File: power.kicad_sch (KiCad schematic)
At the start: 29 parts, among them Q1 DMN3008SFG, Q2 DMN3008SFG, U1 AP33771, U2 AP62150WU, U5 MCP1727T-3302E/SN

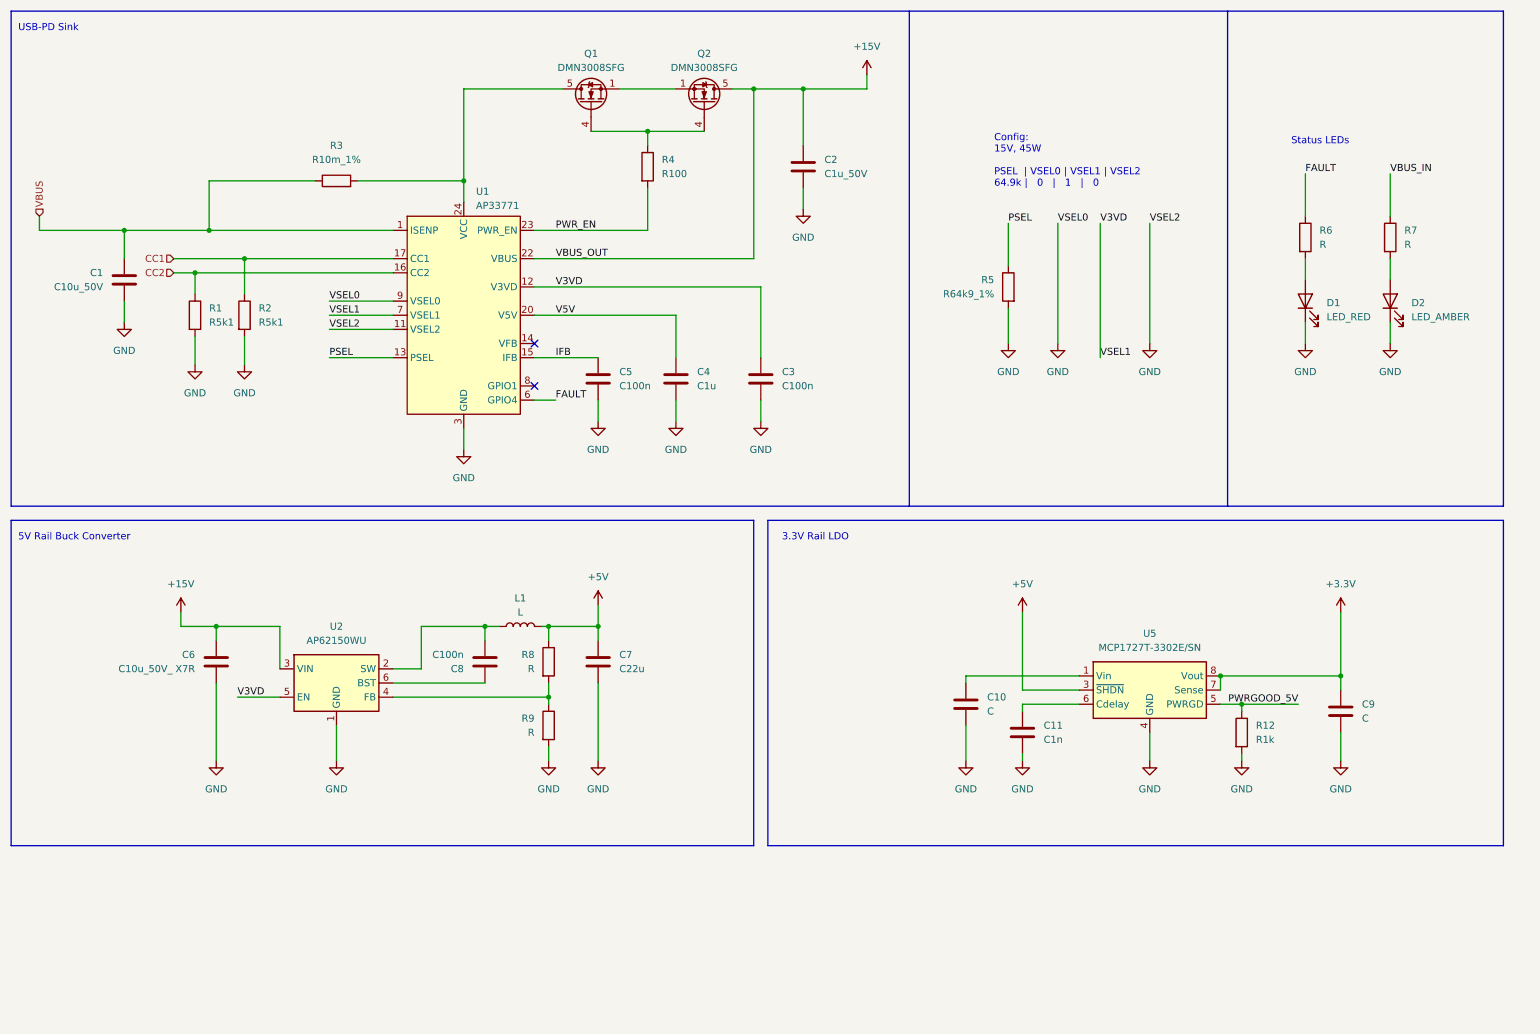
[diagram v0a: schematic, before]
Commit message: Finish first design
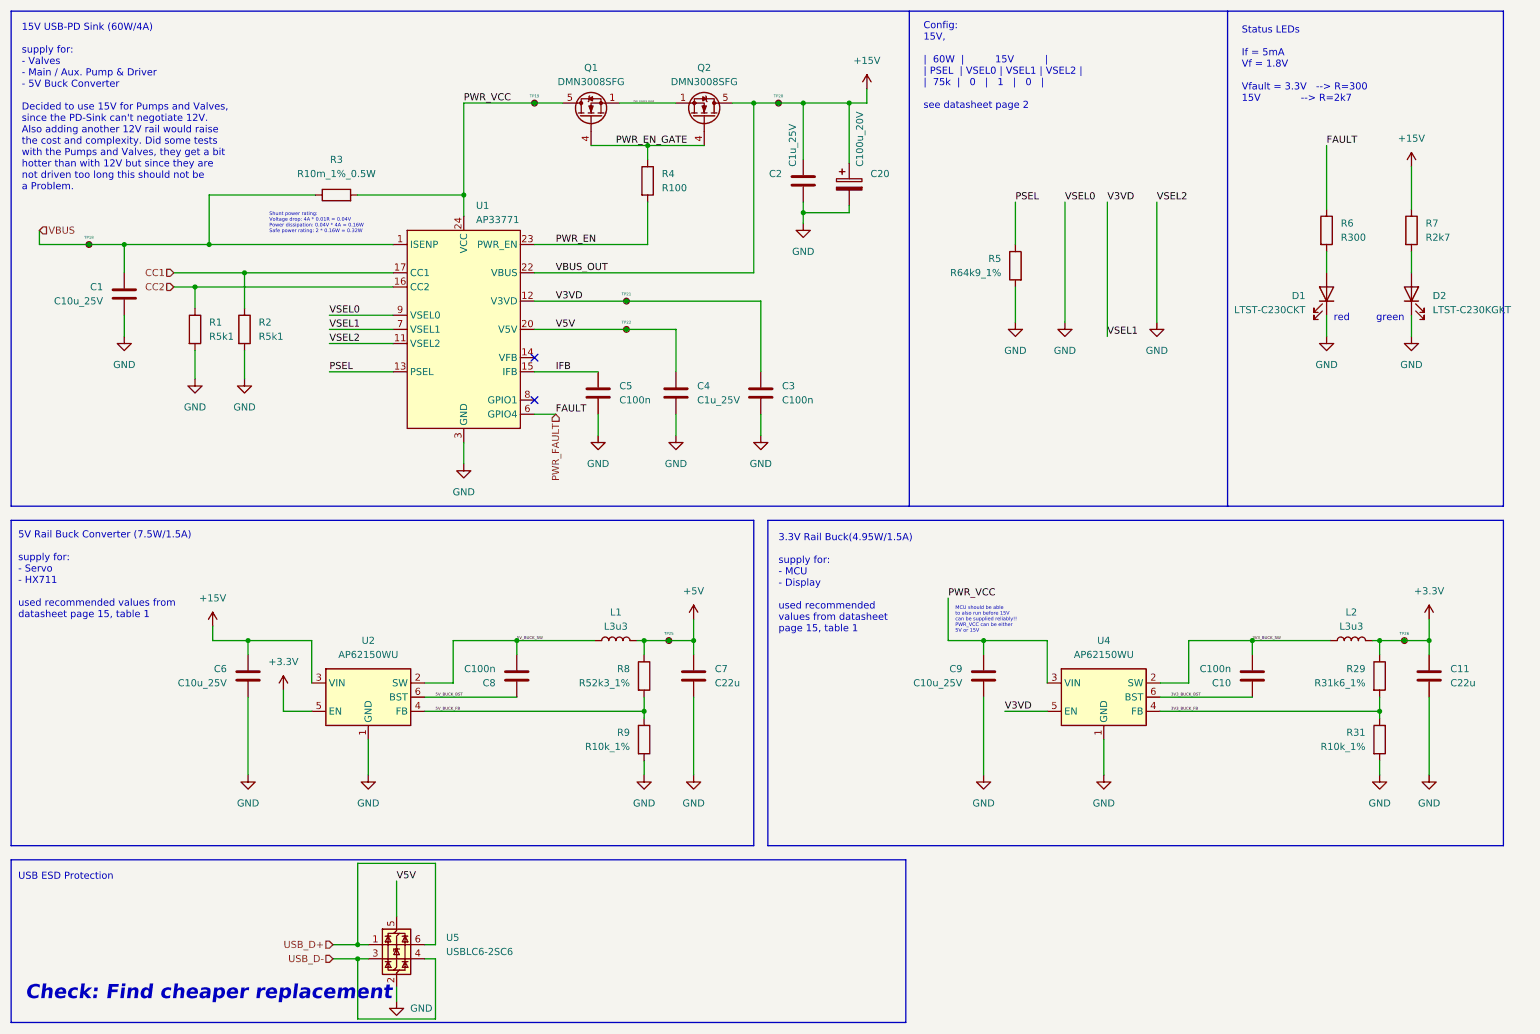
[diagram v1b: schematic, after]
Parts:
- removed R12: R1k, symbol Device:R
- removed U5: MCP1727T-3302E/SN, Package_SO:SOIC-8_3.9x4.9mm_P1.27mm, symbol Regulator_Linear:MCP1727-3302xSN
- added C20: C100u_20V, Capacitor_SMD:CP_Elec_6.3x5.9, symbol Device:C_Polarized
- added L2: L3u3, Inductor_SMD:L_Coilcraft_LPS4018, symbol Device:L
- added R29: R31k6_1%, Resistor_SMD:R_0805_2012Metric, symbol Device:R
- added R31: R10k_1%, Resistor_SMD:R_0805_2012Metric, symbol Device:R
- added TP18, TP19, TP20, TP21, TP22, TP25, TP26: TestPoint_Small, TestPoint:TestPoint_Pad_D1.5mm, symbol Connector:TestPoint_Small
- added U4: AP62150WU, Package_TO_SOT_SMD:TSOT-23-6, symbol Regulator_Switching:AP62150WU
- added U5: USBLC6-2SC6, Package_TO_SOT_SMD:SOT-23-6, symbol Power_Protection:USBLC6-2SC6
- C1: value C10u_50V -> C10u_25V; footprint (none) -> Capacitor_SMD:C_0603_1608Metric; Mouser Part Number (none) -> 81-GRM188R61E106KA3J
- C10: value C -> C100n; footprint (none) -> Capacitor_SMD:C_0603_1608Metric; Mouser Part Number (none) -> 80-C0603C104K3R7867
- C11: value C1n -> C22u; footprint (none) -> Capacitor_SMD:C_0805_2012Metric; Mouser Part Number (none) -> 187-CL21A226MQQNNNF
- C2: value C1u_50V -> C1u_25V; footprint (none) -> Capacitor_SMD:C_0603_1608Metric; Mouser Part Number (none) -> 963-TMK107B7105MA-T
- C3, C5, C8: footprint (none) -> Capacitor_SMD:C_0603_1608Metric; Mouser Part Number (none) -> 80-C0603C104K3R7867
- C4: value C1u -> C1u_25V; footprint (none) -> Capacitor_SMD:C_0603_1608Metric; Mouser Part Number (none) -> 963-TMK107B7105MA-T
- C6: value C10u_50V_ X7R -> C10u_25V; footprint (none) -> Capacitor_SMD:C_0603_1608Metric; Mouser Part Number (none) -> 81-GRM188R61E106KA3J
- C7: footprint (none) -> Capacitor_SMD:C_0805_2012Metric; Mouser Part Number (none) -> 187-CL21A226MQQNNNF
- C9: value C -> C10u_25V; footprint (none) -> Capacitor_SMD:C_0603_1608Metric; Mouser Part Number (none) -> 81-GRM188R61E106KA3J
- D1: value LED_RED -> LTST-C230CKT; footprint (none) -> project:LTST-C230; Mouser Part Number (none) -> 859-LTST-C230CKT
- D2: value LED_AMBER -> LTST-C230KGKT; footprint (none) -> project:LTST-C230; Mouser Part Number (none) -> 859-LTST-C230KGKT
- L1: value L -> L3u3; footprint (none) -> Inductor_SMD:L_Coilcraft_LPS4018; Mouser Part Number (none) -> 994-LPS4018-332MRC
- Q1, Q2: Mouser Part Number (none) -> 621-DMN3008SFG-7
- R1, R2: footprint (none) -> Resistor_SMD:R_0603_1608Metric; Mouser Part Number (none) -> 667-ERJ-3EKF5101V
- R3: value R10m_1% -> R10m_1%_0.5W; footprint (none) -> Resistor_SMD:R_1206_3216Metric; Mouser Part Number (none) -> 504-MFL1206R0100FS
- R4: footprint (none) -> Resistor_SMD:R_0603_1608Metric; Mouser Part Number (none) -> 279-CRG0603F100R
- R5: footprint (none) -> Resistor_SMD:R_0603_1608Metric; Mouser Part Number (none) -> 603-RC0603FR-0764K9P
- R6: value R -> R300; footprint (none) -> Resistor_SMD:R_0805_2012Metric; Mouser Part Number (none) -> 791-WR08X3000FTL
- R7: value R -> R2k7; footprint (none) -> Resistor_SMD:R_0805_2012Metric; Mouser Part Number (none) -> 279-CRGCQ0805F2K7
- R8: value R -> R52k3_1%; footprint (none) -> Resistor_SMD:R_0805_2012Metric; Mouser Part Number (none) -> 652-CR0805FX-5232ELF
- R9: value R -> R10k_1%; footprint (none) -> Resistor_SMD:R_0805_2012Metric; Mouser Part Number (none) -> 71-CRCW0805-10K-E3
- U1: Mouser Part Number (none) -> 621-AP33771DKZ-13
- U2: Mouser Part Number (none) -> 621-AP62150WU-7
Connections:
- net VBUS_IN is gone; now on net +15V: R7.1
- net +15V: now also C20.1, TP20.1
- net +3.3V: now also C11.1, U2.5 (EN), L2.2, R29.1, TP26.1; no longer C9.1
- net +5V: now also TP25.1
- net GND: now also C20.2, R31.2, U4.1 (GND), U5.2 (GND); no longer C10.2
- net V3VD: now also TP21.1, U4.5 (EN); no longer U2.5 (EN)
- net V5V: now also TP22.1, U5.5 (VBUS)
- net VBUS: now also TP18.1
- net 5V_BUCK_SW: now reaches C8.1, L1.1, U2.2 (SW)
- net 5V_BUCK_FB: now reaches R8.2, R9.1, U2.4 (FB)
- net PWR_EN_GATE: now reaches Q1.4 (G), Q2.4 (G), R4.1
- net 3V3_BUCK_SW: now reaches C10.1
- net 3V3_BUCK_SW: now also L2.1, U4.2 (SW)
- net 5V_BUCK_BST: now reaches C8.2, U2.6 (BST)
- net PWR_SOURCE_DRAIN: now reaches Q1.1 (S), Q1.2 (S), Q1.3 (S), Q2.1 (S), Q2.2 (S), Q2.3 (S)
- net PWR_VCC: now reaches Q1.5 (D), R3.2, U1.24 (VCC)
- net PWR_VCC: now also C9.1, TP19.1, U4.3 (VIN)
- net FAULT renamed PWR_FAULT
- new net 3V3_BUCK_BST: C10.2, U4.6 (BST)
- new net 3V3_BUCK_FB: R29.2, R31.1, U4.4 (FB)
- new net USB_D+: U5.1 (I/O1), U5.6 (I/O1)
- new net USB_D-: U5.3 (I/O2), U5.4 (I/O2)
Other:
- note added: "15V USB-PD Sink (60W/4A) supply for: - Valves - Main / Aux. Pump & Driver - 5V Buck Converter Decided to use 15V for Pumps and Valves, since the PD-Sink can't negotiate 12V. Also adding another 12V rail would raise the cost and complexity. Did some tests with the Pumps and Valves, they get a bit hotter than with 12V but since they are not driven too long this should not be a Problem."
- note added: "3.3V Rail Buck(4.95W/1.5A) supply for: - MCU - Display used recommended values from datasheet page 15, table 1"
- note added: "5V Rail Buck Converter (7.5W/1.5A) supply for: - Servo - HX711 used recommended values from datasheet page 15, table 1"
- note added: "Check: Find cheaper replacement"
- note added: "Config: 15V, | 60W | 15V | | PSEL | VSEL0 | VSEL1 | VSEL2 | | 75k | 0 | 1 | 0 | see datasheet page 2"
- note added: "MCU should be able to also run before 15V can be supplied reliably!! PWR_VCC can be either 5V or 15V"
- note added: "Shunt power rating: Voltage drop: 4A * 0.01R = 0.04V Power dissipation: 0.04V * 4A = 0.16W Safe power rating: 2 * 0.16W = 0.32W"
- note added: "Status LEDs If = 5mA Vf = 1.8V Vfault = 3.3V --> R=300 15V --> R=2k7"
- note added: "USB ESD Protection"
- note added: "green"
- note added: "red"
- note removed: "3.3V Rail LDO"
- note removed: "5V Rail Buck Converter"
- note removed: "Config: 15V, 45W PSEL | VSEL0 | VSEL1 | VSEL2 64.9k | 0 | 1 | 0"
- note removed: "Status LEDs"
- note removed: "USB-PD Sink"
- moved on the sheet: C1, C2, C3, C4, C5, C6, C7, C8, D1, D2, L1, Q1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
